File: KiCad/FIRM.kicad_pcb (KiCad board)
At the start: 4 copper layers, 38.5 x 38.5 mm, 98 parts, among them J1 Conn_01x02_Pin, J2 DM3CS-SF, Q2 IRLML6402, SW1 PTS815, U1 STM32F405RGTx, U2 MIC5219-3.3YM5, U6 A-USBC-20F0-EA-GSR05, U7 W25Q128JVS, X2 32.768khz, Y1 12 MHz

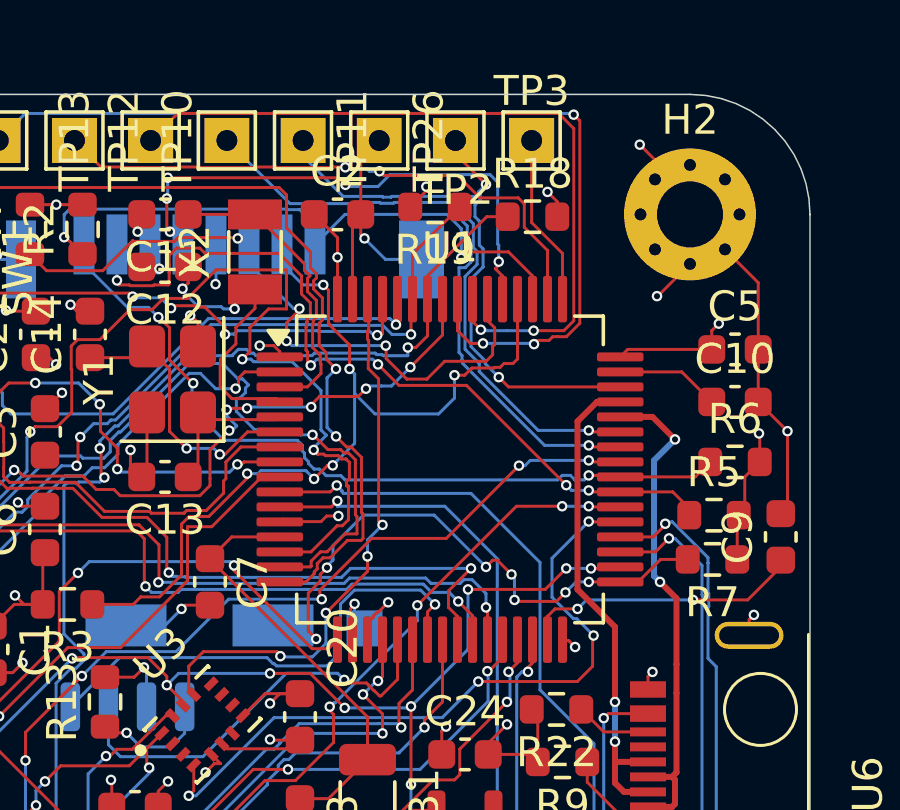
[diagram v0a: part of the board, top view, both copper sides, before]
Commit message: backup
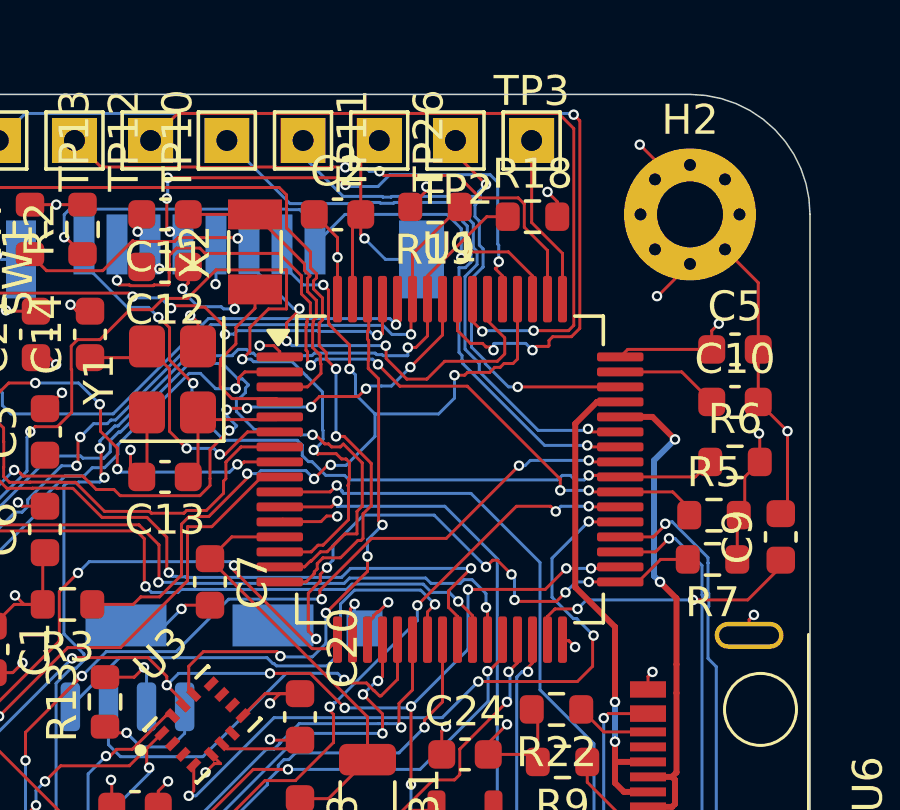
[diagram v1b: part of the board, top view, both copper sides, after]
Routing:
- net /SDIO_D3: track 29.9 -> 29.1 mm
- net /PB4: track 32.2 -> 32.9 mm

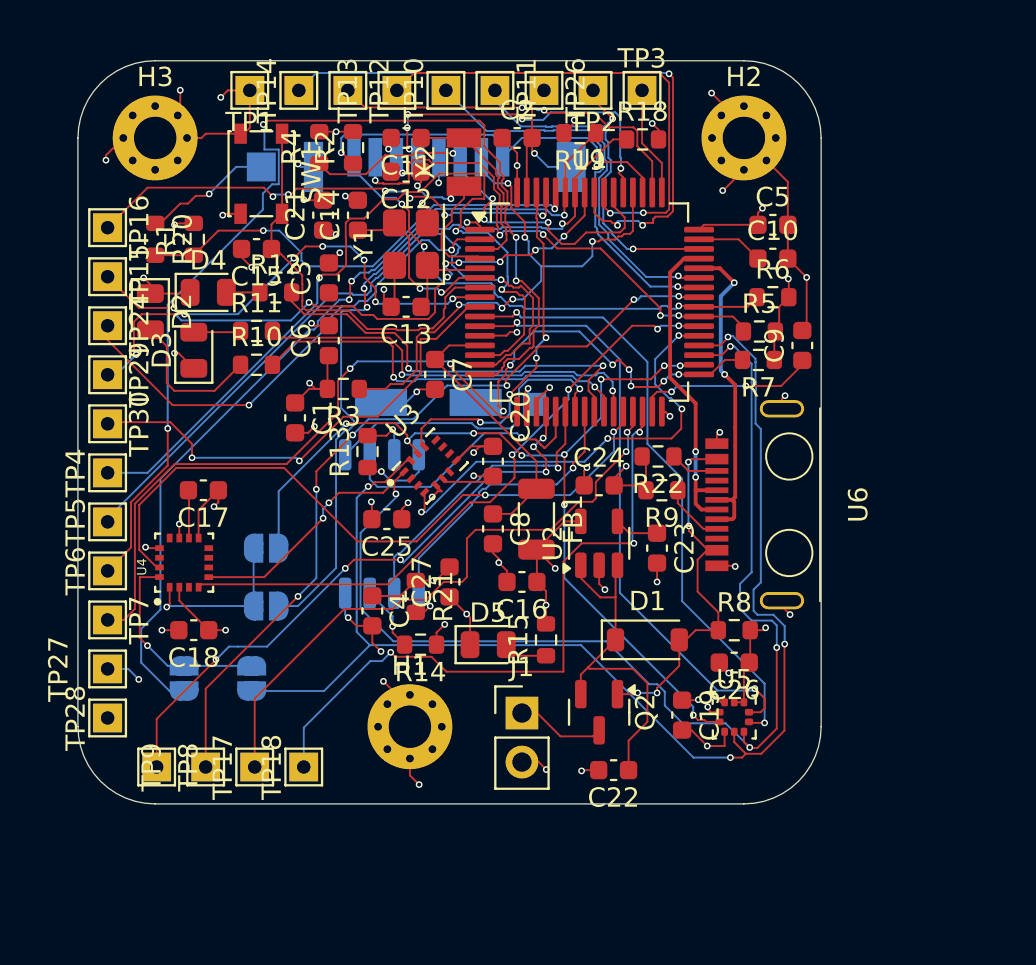
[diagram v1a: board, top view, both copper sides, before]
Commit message: almost done
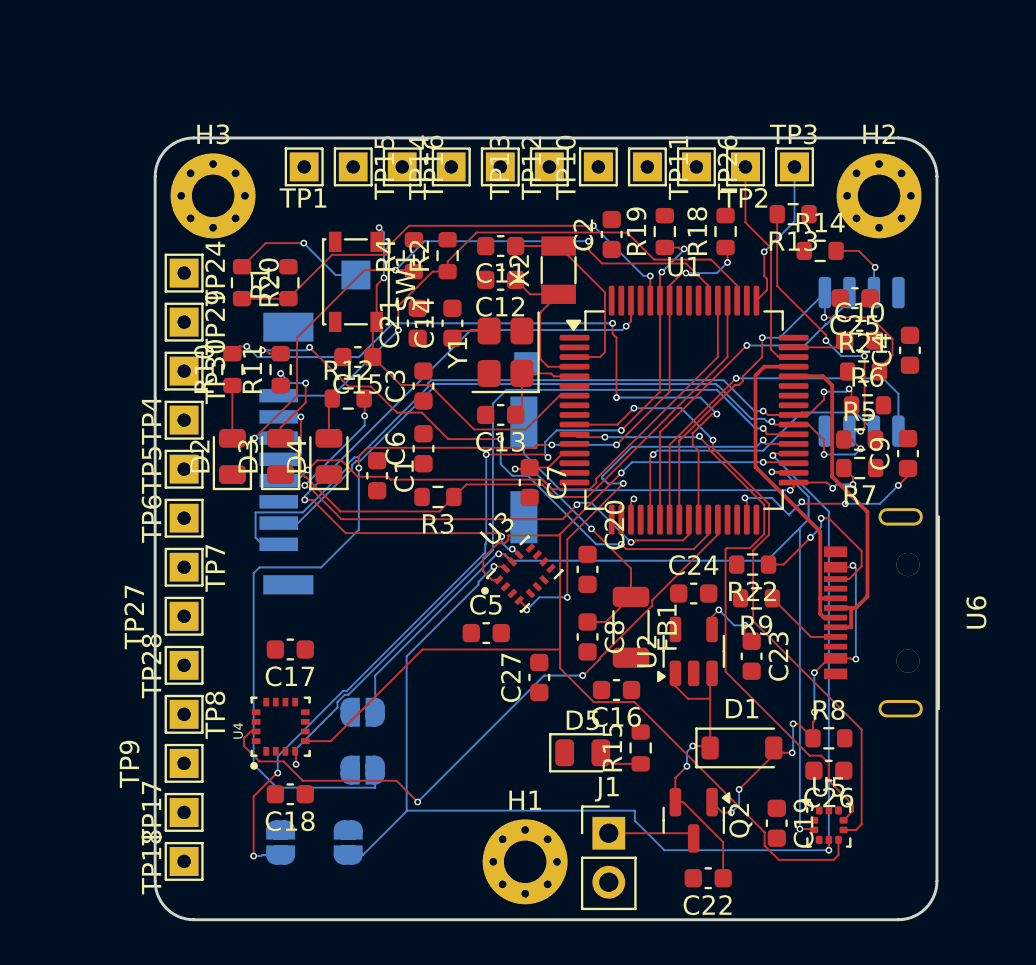
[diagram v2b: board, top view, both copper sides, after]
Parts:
- moved C4 30.9 mm to (139.1, 111.0), turned to 90 degrees
- moved R14 29.1 mm to (134.4, 105.8), turned to 0 degrees
- moved C25 26.8 mm to (136.2, 108.3)
- moved U7 26.2 mm to (136.6, 111.6), turned to -90 degrees
- moved R21 26.0 mm to (136.7, 112.1), turned to 0 degrees
- moved C5 25.8 mm to (117.2, 125.7)
- moved R13 25.2 mm to (133.1, 104.0), turned to 180 degrees
- moved TP16 15.6 mm to (112.8, 101.5)
- moved TP15 13.9 mm to (110.3, 101.5)
- moved D4 10.6 mm to (109.0, 116.5), turned to 90 degrees
- moved C18 9.86 mm to (107.0, 134.0)
- moved JP1 9.86 mm to (106.5, 136.5)
- moved JP2 9.86 mm to (110.0, 136.5)
- moved JP3 9.86 mm to (110.8, 132.8)
- moved JP4 9.86 mm to (110.8, 129.8)
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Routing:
- net GND: track 107.1 -> 0.00 mm, vias 48 -> 0
- net +3.3V: track 59.1 -> 1.14 mm, vias 27 -> 1
- net /PA2: track 56.0 -> 0.00 mm, vias 4 -> 0
- net /PA0: track 43.2 -> 0.00 mm, vias 3 -> 0
- net /PA8: track 41.6 -> 0.00 mm, vias 6 -> 0
- net /PA1: track 36.7 -> 0.00 mm, vias 1 -> 0
- net /PB11: track 34.5 -> 0.00 mm, vias 3 -> 0
- net /PB4: track 32.9 -> 0.00 mm, vias 3 -> 0
- net /PA3: track 32.3 -> 0.00 mm, vias 2 -> 0
- net /PB10: track 32.0 -> 0.00 mm, vias 2 -> 0
- net /PA4: track 31.8 -> 0.00 mm, vias 6 -> 0
- net /PB5: track 31.5 -> 0.00 mm, vias 8 -> 0
- net /PB8: track 26.0 -> 0.00 mm, vias 6 -> 0
- net /PC13: track 25.9 -> 0.00 mm, vias 2 -> 0
- net /PB3: track 25.6 -> 0.00 mm, vias 2 -> 0
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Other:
- board size 38.5 x 38.5 mm -> 40.5 x 40.5 mm

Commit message: chat we are so back
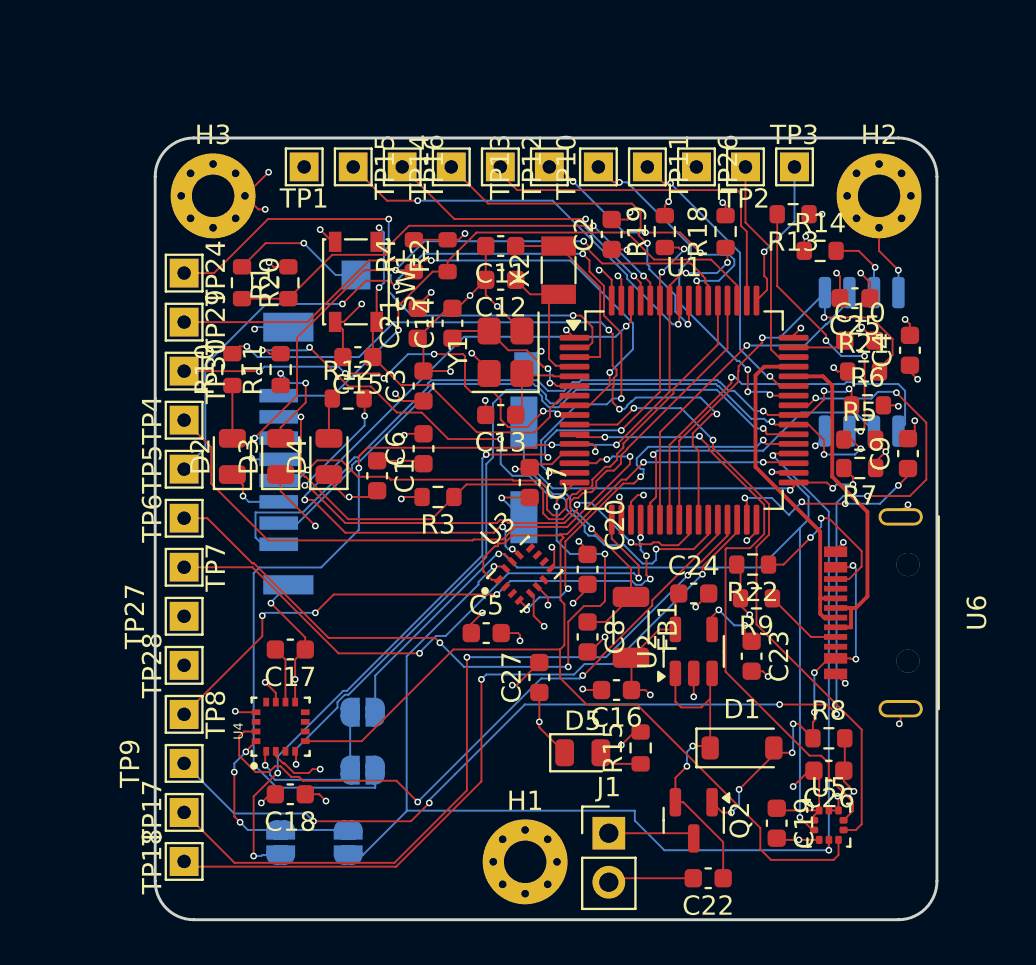
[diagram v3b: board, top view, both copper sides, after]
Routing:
- net GND: track 0.00 -> 96.1 mm, vias 0 -> 47
- net /PA8: track 0.00 -> 64.7 mm, vias 0 -> 7
- net +3.3V: track 1.14 -> 55.3 mm, vias 1 -> 33
- net /PA1: track 0.00 -> 44.8 mm, vias 0 -> 5
- net /PB10: track 0.00 -> 41.1 mm, vias 0 -> 2
- net /PB11: track 0.00 -> 39.9 mm, vias 0 -> 2
- net /PA2: track 0.00 -> 36.4 mm, vias 0 -> 4
- net /PC0: track 0.00 -> 31.9 mm, vias 0 -> 2
- net /PA0: track 0.00 -> 31.8 mm, vias 0 -> 2
- net /PA4: track 0.00 -> 31.3 mm, vias 0 -> 6
- net /PA3: track 0.00 -> 30.9 mm, vias 0 -> 2
- net /PC13: track 0.00 -> 28.8 mm, vias 0 -> 2
- net /PC1: track 0.00 -> 24.6 mm, vias 0 -> 6
- net /PB5: track 0.00 -> 21.6 mm, vias 0 -> 2
- net /PB4: track 0.00 -> 19.0 mm, vias 0 -> 2
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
